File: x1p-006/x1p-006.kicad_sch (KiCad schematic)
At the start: 11 parts, among them U1 AD24C02, U3 TLP172GM(TPL,E(O, U6 TLP172GM(TPL,E(O

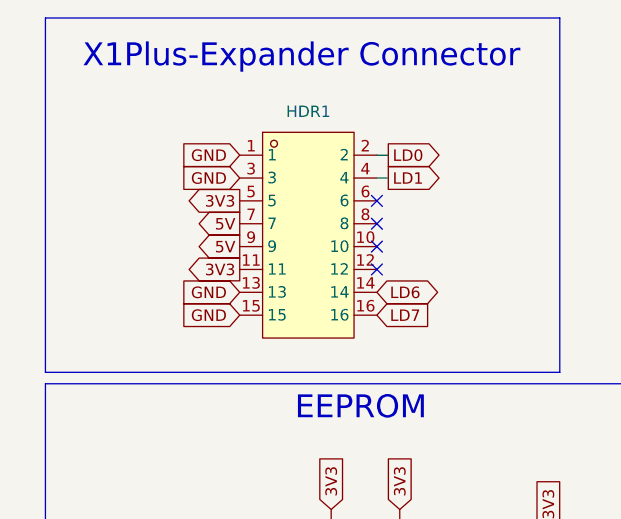
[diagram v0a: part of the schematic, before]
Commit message: 0 drc errors \o/
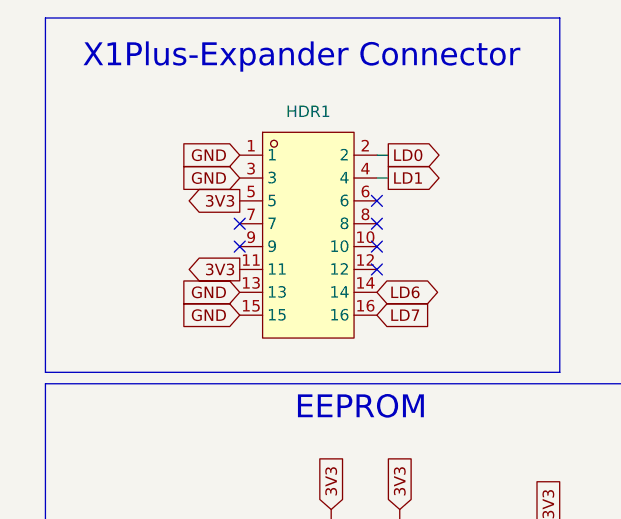
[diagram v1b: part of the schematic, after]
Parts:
- C1: footprint x1p-005:C0402 -> x1p-006:C0402
- HDR1: footprint x1p-005:HDR-TH_16P-P2.54-H-F-R2-C8-W8.5 -> x1p-006:HDR-TH_16P-P2.54-H-F-R2-C8-W8.5
- R1, R2: footprint x1p-005:R0402 -> x1p-006:R0402
- U1: footprint x1p-005:SOT-23-5_L2.9-W1.6-P0.95-LS2.8-BL -> x1p-006:SOT-23-5_L2.9-W1.6-P0.95-LS2.8-BL
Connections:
- net 5V: no longer names the net of HDR1.7
- net 5V: no longer HDR1.9
- no-connect marks 4 -> 6

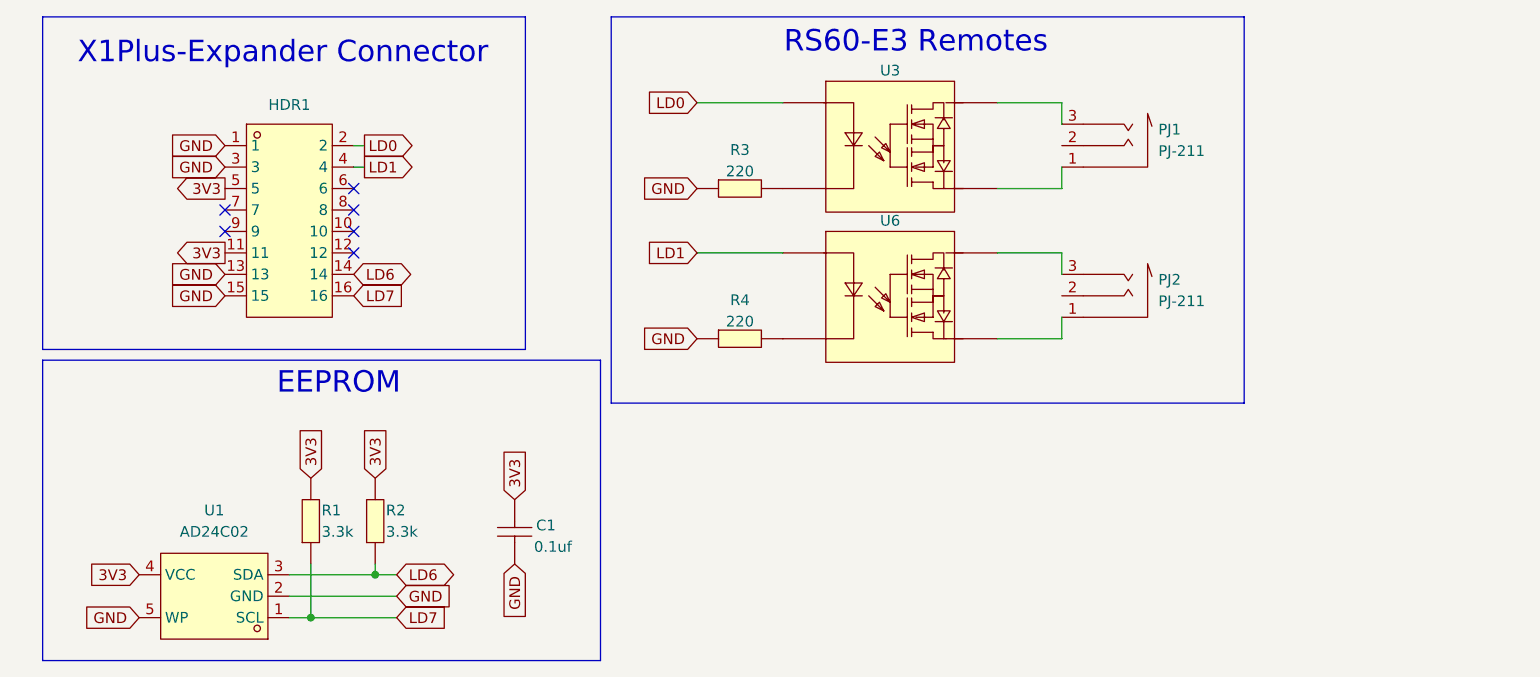
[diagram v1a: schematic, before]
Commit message: x1p-006-b01
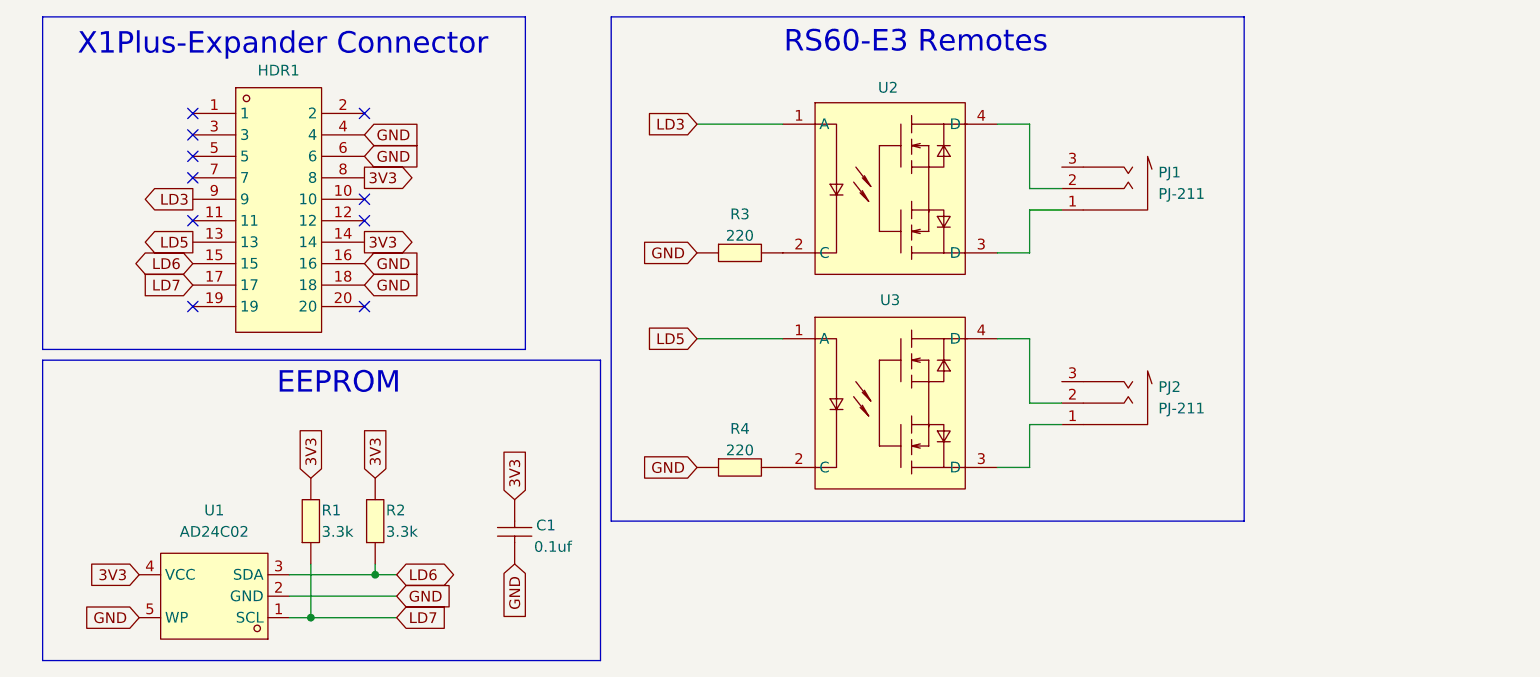
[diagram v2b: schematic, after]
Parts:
- removed HDR1: PM254-2-08-W-8.5, x1p-006:HDR-TH_16P-P2.54-H-F-R2-C8-W8.5, symbol lcsc:PM254-2-08-W-8.5
- removed U3, U6: TLP172GM(TPL,E(O, x1p-006:SMD-4_L4.6-W3.7-P2.54-LS7.0-BR, symbol x1p-006:TLP172GM(TPL,E(O
- added HDR1: 220R-2*10P H=8.5MM Ytype Gold-plated black, x1p-006:HDR-TH_20P-P2.54-H-F-R2-C10-S2.54-W10.2, symbol x1p-006:220R-2*10PH=8.5MMYtypeGold-platedblack
- added U2, U3: TLP240A(TP1,F, x1p-006:RELAY-SMD_TLP240A, symbol x1p-006:TLP240A(TP1,F
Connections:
- net 3V3: now also HDR1.14, HDR1.8
- net GND: now also HDR1.16, HDR1.18, HDR1.4, HDR1.6
- net LD6: now also HDR1.15
- net LD7: now also HDR1.17
- net at R4.2: now also U3.2 (C)
- net at PJ2.1: now also U3.3 (D)
- net at PJ1.1: now also U2.3 (D)
- net at PJ1.2: now also U2.4 (D)
- net at R3.2: now also U2.2 (C)
- net at PJ2.2: now also U3.4 (D)
- new net LD3: HDR1.9, U2.1 (A)
- new net LD5: HDR1.13, U3.1 (A)
- no-connect marks 6 -> 10

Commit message: change jack to trrs
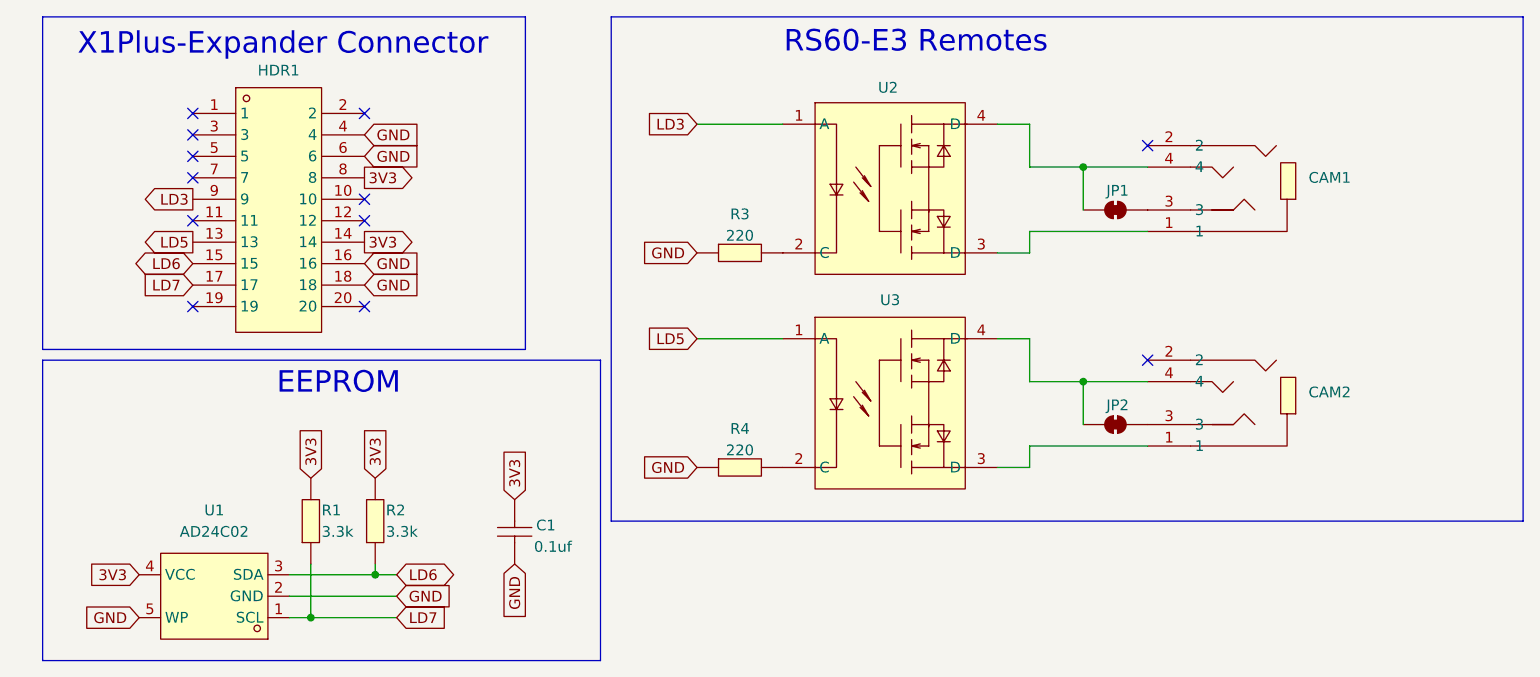
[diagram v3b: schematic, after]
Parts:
- removed PJ1, PJ2: PJ-211, x1p-006:AUDIO-TH_PJ-211, symbol x1p-006:PJ-211
- added CAM1, CAM2: PJ-2013-L6S, x1p-006:AUDIO-TH_PJ-2013-L6S, symbol x1p-006:PJ-2013-L6S
- added JP1, JP2: SolderJumper_2_Bridged, Jumper:SolderJumper-2_P1.3mm_Bridged_RoundedPad1.0x1.5mm, symbol Jumper:SolderJumper_2_Bridged
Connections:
- net at U2.3 (D): now also CAM1.1
- net at U2.4 (D): now also CAM1.4, JP1.1 (A)
- net at U3.3 (D): now also CAM2.1
- net at U3.4 (D): now also CAM2.4, JP2.1 (A)
- new net: CAM2.3, JP2.2 (B)
- new net: CAM1.3, JP1.2 (B)
- no-connect marks 10 -> 12

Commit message: fixes
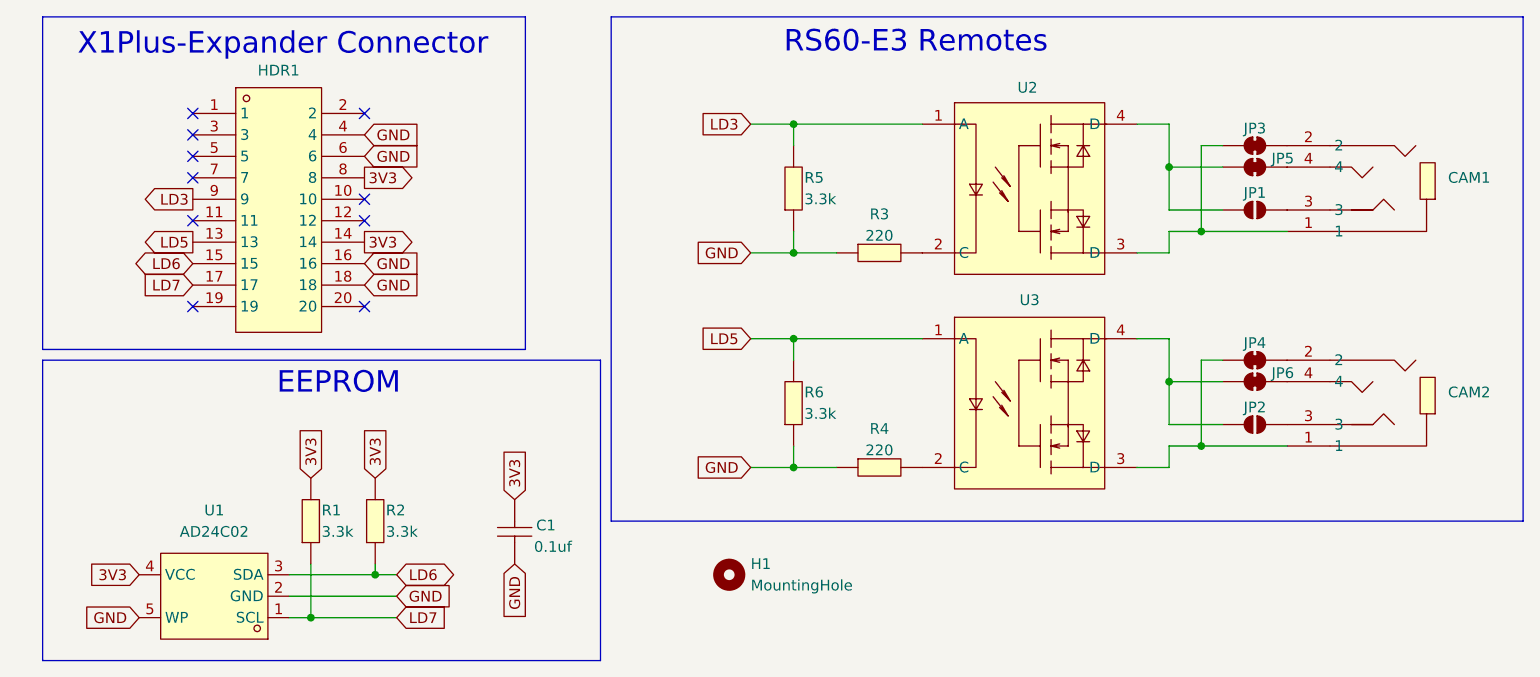
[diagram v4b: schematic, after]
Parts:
- removed JP1, JP2: SolderJumper_2_Bridged, Jumper:SolderJumper-2_P1.3mm_Bridged_RoundedPad1.0x1.5mm, symbol Jumper:SolderJumper_2_Bridged
- added H1: MountingHole, MountingHole:MountingHole_2.2mm_M2_ISO7380, symbol Mechanical:MountingHole
- added JP1, JP2: SolderJumper_2_Open, Jumper:SolderJumper-2_P1.3mm_Open_RoundedPad1.0x1.5mm, symbol Jumper:SolderJumper_2_Open
- added JP3, JP4, JP5, JP6: SolderJumper_2_Bridged, Jumper:SolderJumper-2_P1.3mm_Bridged_RoundedPad1.0x1.5mm, symbol Jumper:SolderJumper_2_Bridged
- added R5, R6: 3.3k, x1p-006:R0402, symbol lcsc:0402WGF3301TCE
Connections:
- net GND: now also R5.1, R6.1
- net LD3: now also R5.2
- net LD5: now also R6.2
- net at CAM1.1, U2.3 (D): now also JP3.1 (A)
- net at U2.4 (D): now also JP1.1 (A), JP5.1 (A); no longer CAM1.4
- net at CAM2.1, U3.3 (D): now also JP4.1 (A)
- net at CAM2.2: now also JP4.2 (B)
- net at CAM2.3: now also JP2.2 (B)
- net at U3.4 (D): now also JP2.1 (A), JP6.1 (A); no longer CAM2.4
- net at CAM1.2: now also JP3.2 (B)
- net at CAM1.3: now also JP1.2 (B)
- new net: CAM2.4, JP6.2 (B)
- new net: CAM1.4, JP5.2 (B)
- no-connect marks 12 -> 10
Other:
- moved on the sheet: CAM1, CAM2, R3, R4, U2, U3

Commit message: change to TRS jack, change ssr to instock part, remove jumpers
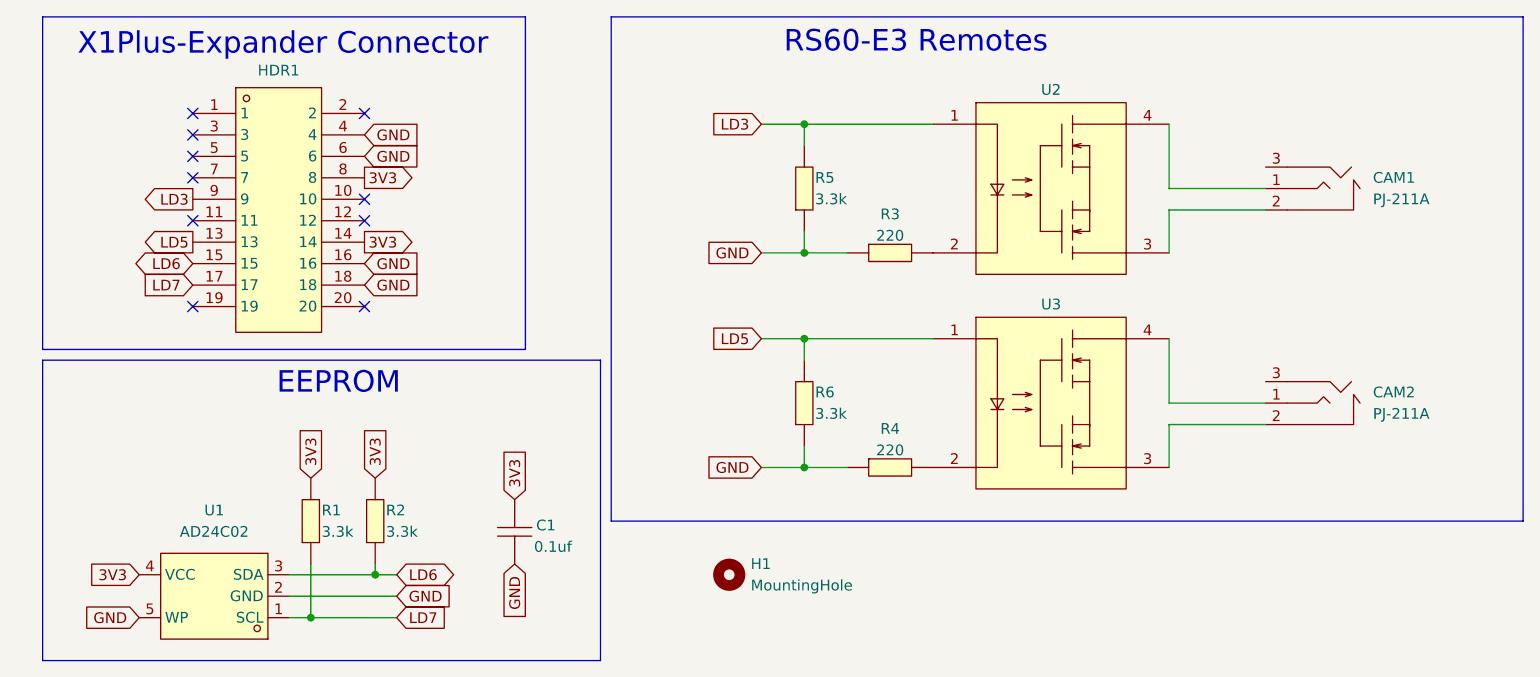
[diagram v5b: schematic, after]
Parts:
- removed CAM1, CAM2: PJ-2013-L6S, x1p-006:AUDIO-TH_PJ-2013-L6S, symbol x1p-006:PJ-2013-L6S
- removed JP1, JP2: SolderJumper_2_Open, Jumper:SolderJumper-2_P1.3mm_Open_RoundedPad1.0x1.5mm, symbol Jumper:SolderJumper_2_Open
- removed JP3, JP4, JP5, JP6: SolderJumper_2_Bridged, Jumper:SolderJumper-2_P1.3mm_Bridged_RoundedPad1.0x1.5mm, symbol Jumper:SolderJumper_2_Bridged
- removed U2, U3: TLP240A(TP1,F, x1p-006:RELAY-SMD_TLP240A, symbol x1p-006:TLP240A(TP1,F
- added CAM1, CAM2: PJ-211A, x1p-006:AUDIO-TH_PJ-211A, symbol x1p-006:PJ-211A
- added U2, U3: AQY212EHAX, x1p-006:SOP-4_L6.5-W4.6-P2.54-LS10.2-TR, symbol x1p-006:AQY212EHAX
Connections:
- net LD3: now also U2.1 (A)
- net LD5: now also U3.1 (A)
- net at R4.2: now also U3.2 (K)
- net at R3.2: now also U2.2 (K)
- new net: CAM1.2, U2.3 (S1)
- new net: CAM1.1, U2.4 (S)
- new net: CAM2.2, U3.3 (S1)
- new net: CAM2.1, U3.4 (S)
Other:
- moved on the sheet: R3, R4, R5, R6
